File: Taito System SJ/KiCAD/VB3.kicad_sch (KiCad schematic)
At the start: 30 parts, among them U13 74LS157, U14 74LS157, U15 74LS175, U19 74LS32, U2 74LS157, U27 74LS273, U28 74LS86, U29 74LS163, U33 74LS27, U39 74LS32, U4 74LS04, U40 74LS174, U41 RAM_5501, U42 74LS86, U43 74LS163, U5 74LS74, U54 74LS10, U55 74LS86, U56 74LS27, U57 74LS163, U6 74LS32, U69 RAM_5501, U7 74LS74, U70 74LS86, U71 74LS163, U72 74LS08

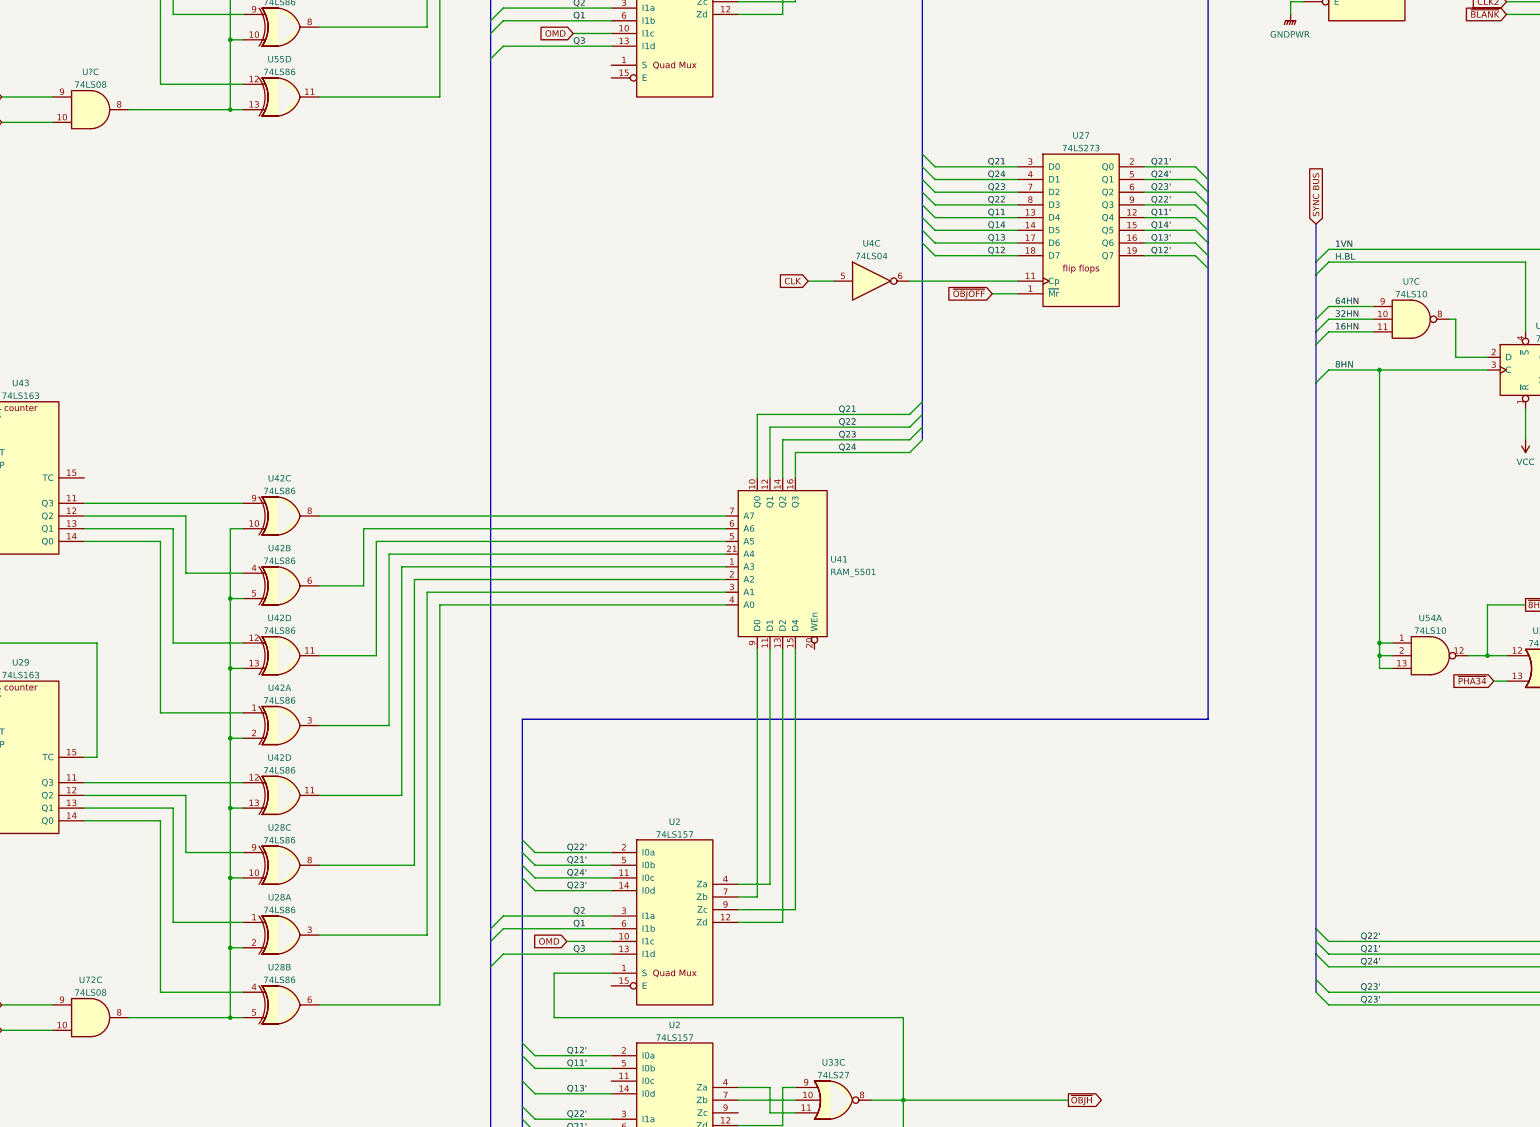
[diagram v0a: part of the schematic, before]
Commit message: Update before transfer
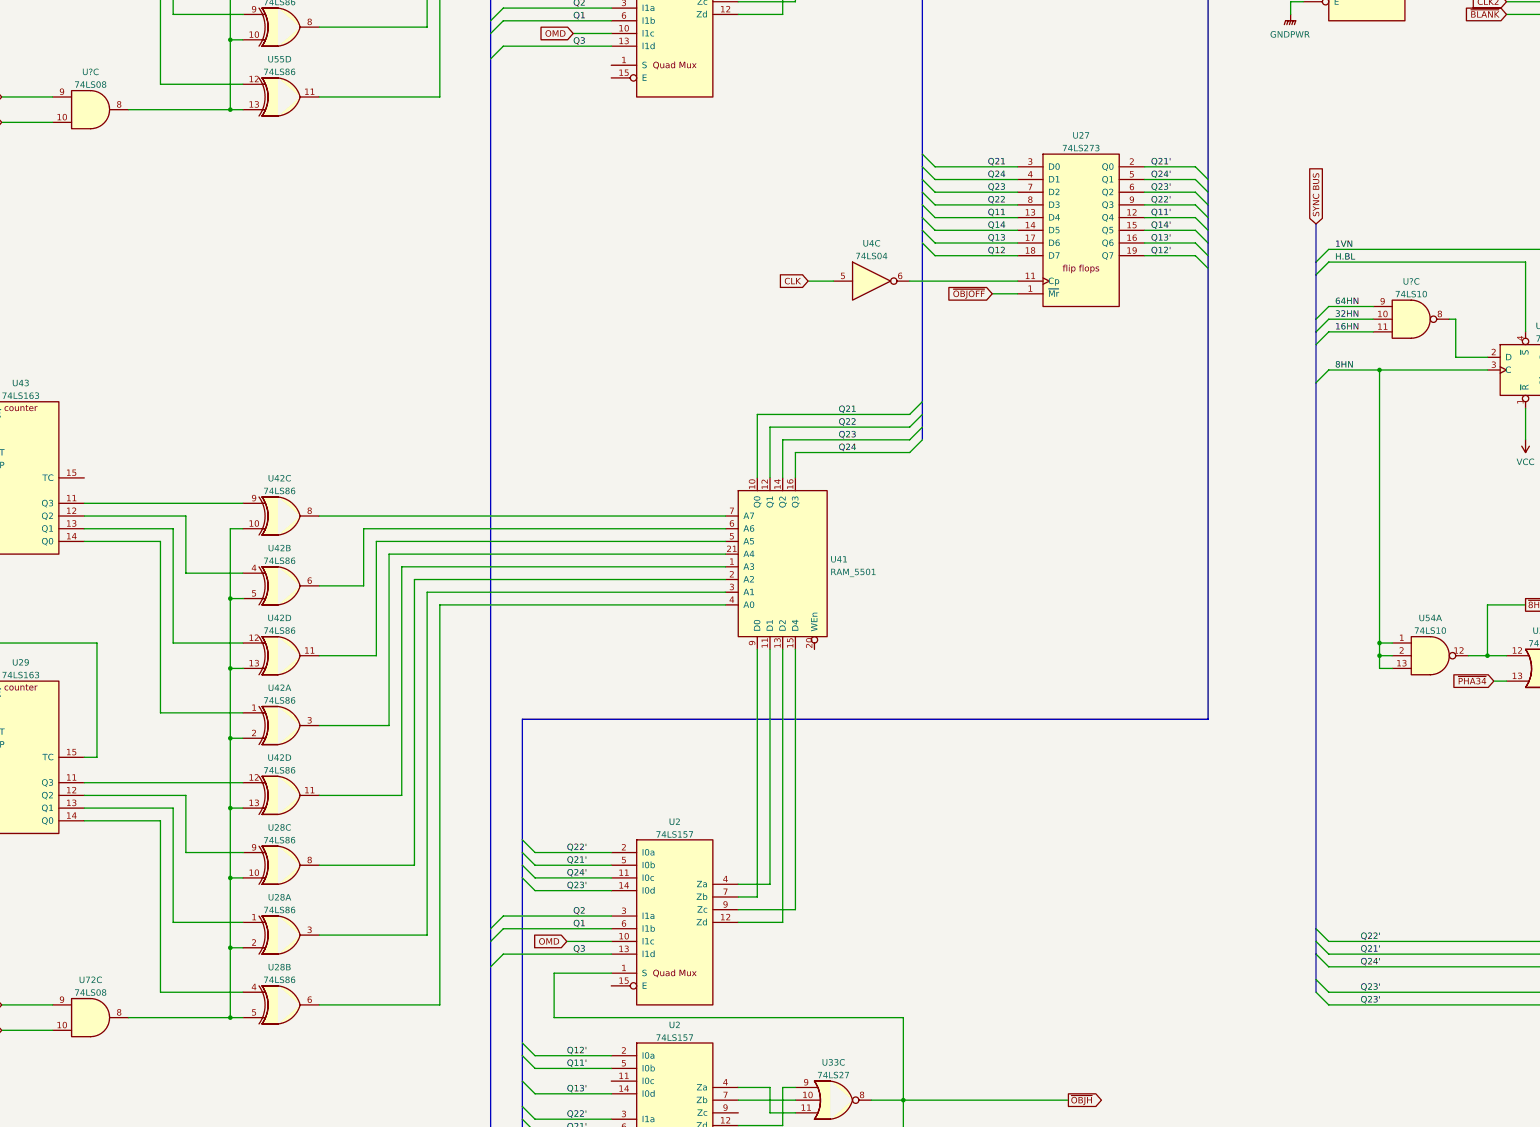
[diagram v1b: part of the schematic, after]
